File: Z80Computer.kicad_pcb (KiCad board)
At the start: 2 copper layers, 152.4 x 129.5 mm, 38 parts, among them IC1 Z80CPU, IC2_EEPROM1 28C256, IC6_SRAM1 KM62256CLP, J1 Conn_Coaxial_Power, J2 Conn_01x08_Pin, J3 Conn_01x08_Pin, SW1 SW_Push, U1 74LS244, U2 74LS32, U3 74LS273, U4 74LS138, U5 74LS00, U6 74LS244, U7 74LS00, X1 CXO_DIP14

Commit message: Added text
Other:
- board text added: "Itch.io https://adrianpilko.itch.io Github https://github.com/AdrianPilko Youtube @byteforever7829"
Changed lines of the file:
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@@
   (gr_line (start 55.88 162.56) (end 58.42 162.56)
     (stroke (width 0.1) (type default)) (layer "Edge.Cuts"))
+  (gr_text "Itch.io  https://adrianpilko.itch.io\nGithub   https://github.com/AdrianPilko\nYoutube  @byteforever7829" (at 165.1 40.64) (layer "Edge.Cuts")
+    (effects (font (size 1 1) (thickness 0.15)) (justify left bottom))
+  )
   (segment (start 53.34 40.64) (end 58.42 40.64) (width 0.25) (layer "F.Cu") (net 1))
   (segment (start 58.42 35.56) (end 58.42 40.64) (width 0.25) (layer "B.Cu") (net 1))

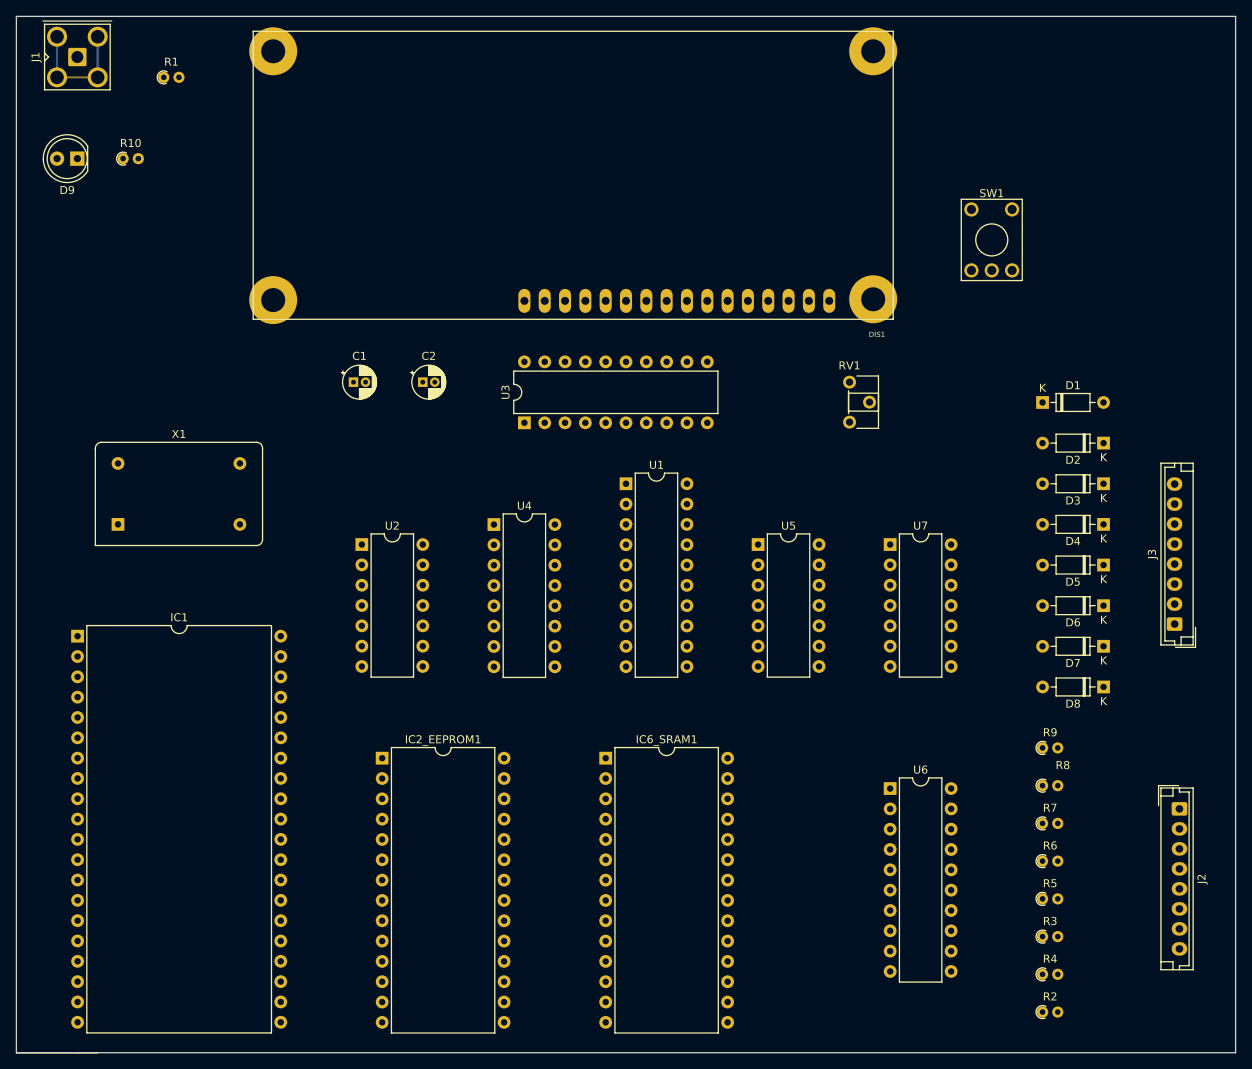
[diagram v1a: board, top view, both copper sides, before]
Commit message: autorouted
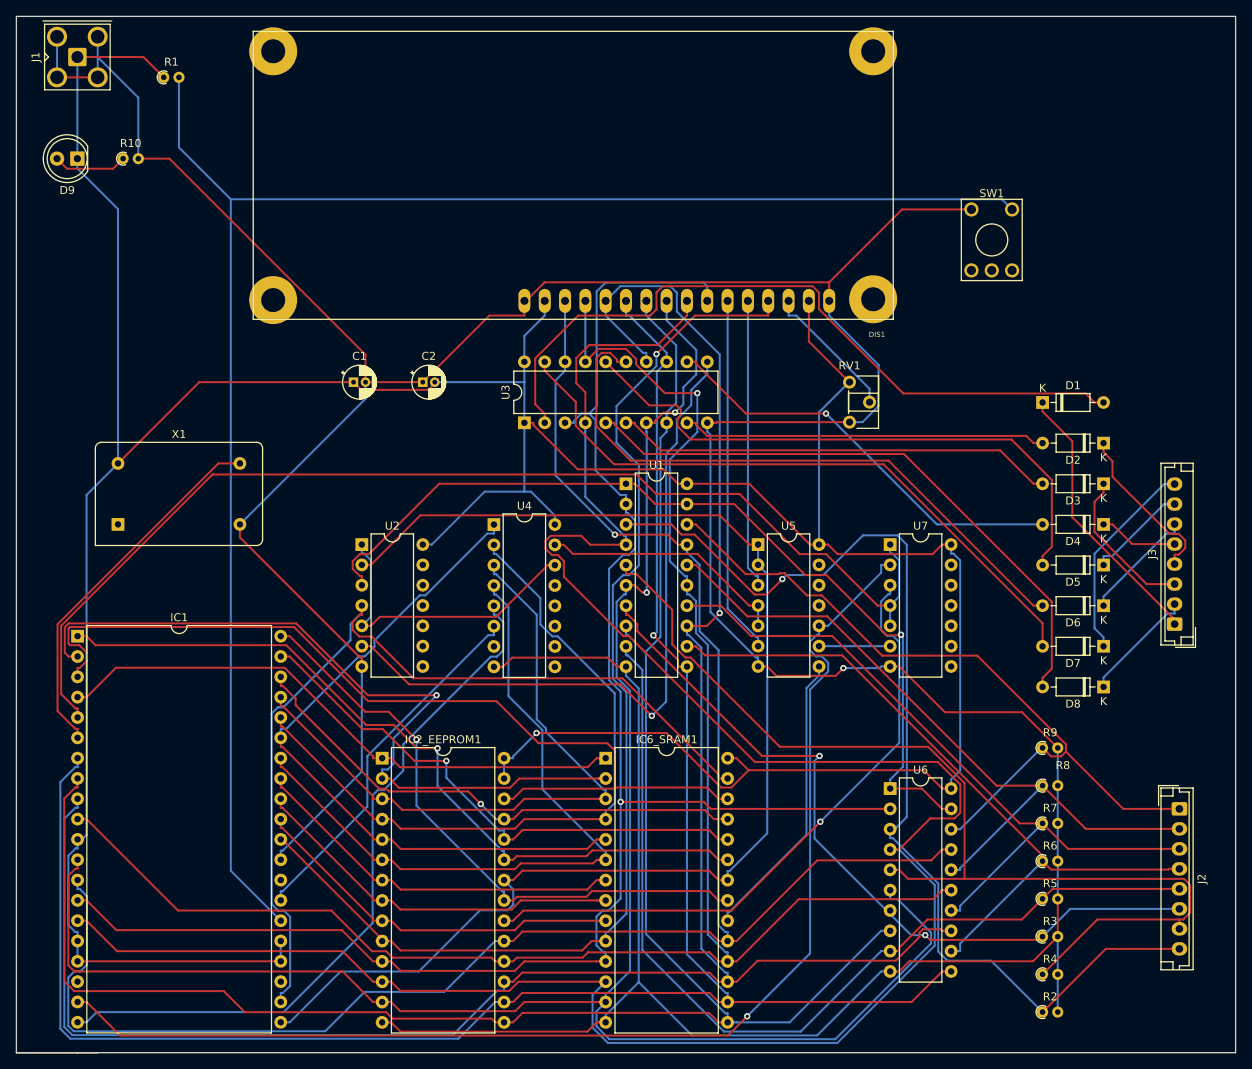
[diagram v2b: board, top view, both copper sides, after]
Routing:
- net Z80_PWRCAP: track 15.2 -> 537.7 mm, vias 0 -> 1
- net +5V: track 0.00 -> 455.6 mm, vias 0 -> 1
- net /D1: track 0.00 -> 275.2 mm
- net /D5: track 0.00 -> 262.0 mm, vias 0 -> 1
- net /D4: track 0.00 -> 246.5 mm, vias 0 -> 1
- net /D2: track 0.00 -> 244.0 mm, vias 0 -> 2
- net /D3: track 0.00 -> 239.5 mm
- net /D7: track 0.00 -> 235.5 mm, vias 0 -> 1
- net /D6: track 0.00 -> 222.1 mm, vias 0 -> 1
- net /D0: track 0.00 -> 215.9 mm, vias 0 -> 1
- net Net-(IC1-~{RESET}): track 0.00 -> 208.9 mm
- net ~{RD}: track 0.00 -> 165.8 mm
- net ~{MREQ}: track 0.00 -> 154.1 mm, vias 0 -> 1
- net /A0: track 0.00 -> 145.2 mm, vias 0 -> 1
- net /A15: track 0.00 -> 142.0 mm
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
